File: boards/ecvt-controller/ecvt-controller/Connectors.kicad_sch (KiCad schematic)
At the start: 8 parts, among them J2 917782-1, J3 917782-1, J4 15311026, J5 917786-1, J6 917780-1

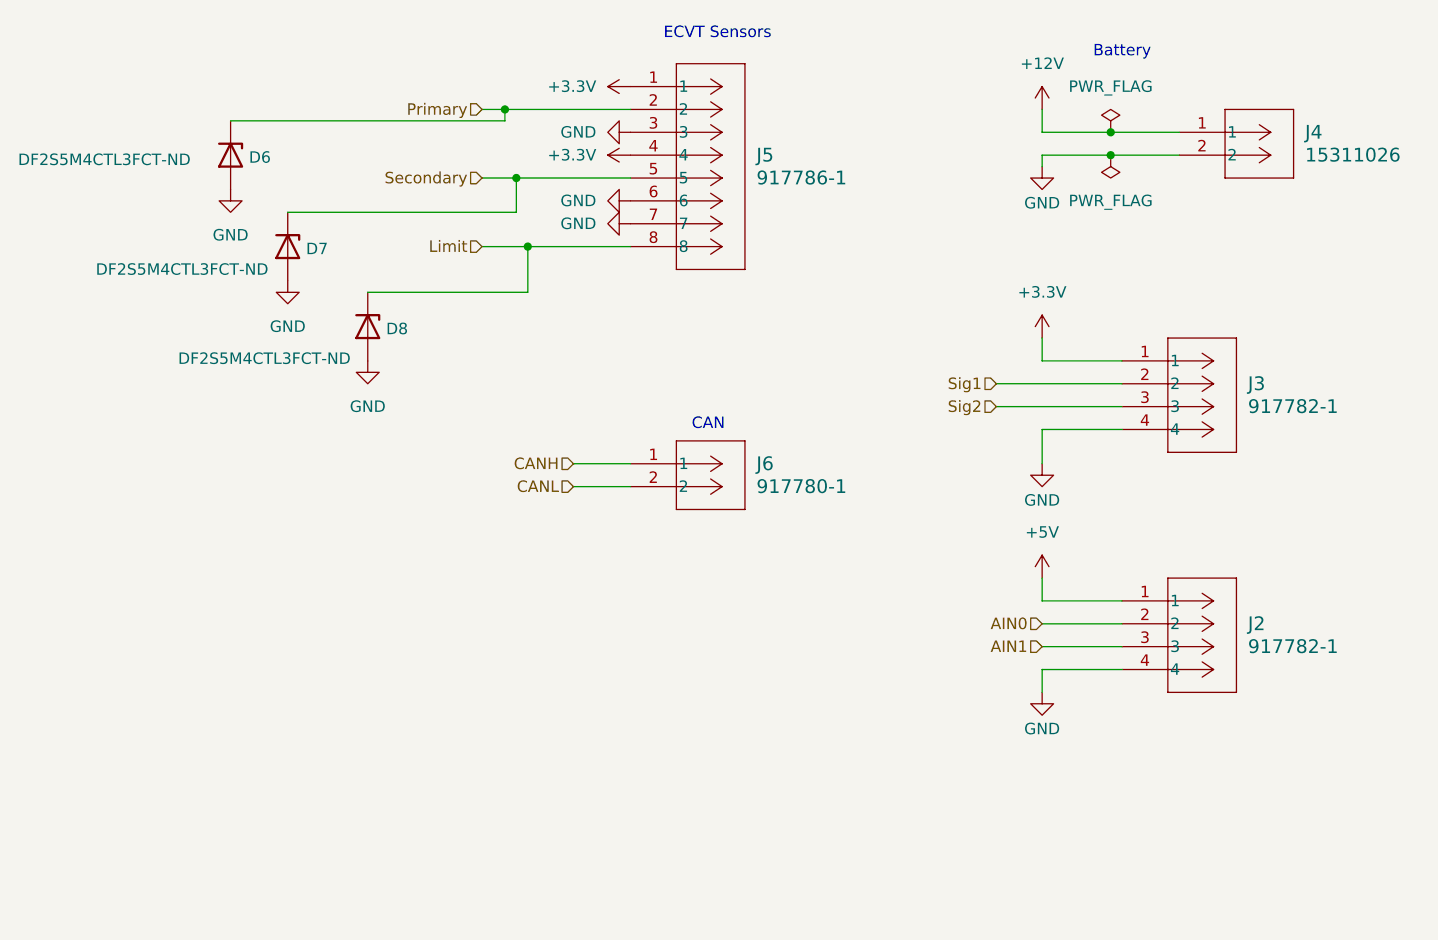
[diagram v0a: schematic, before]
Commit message: almost there
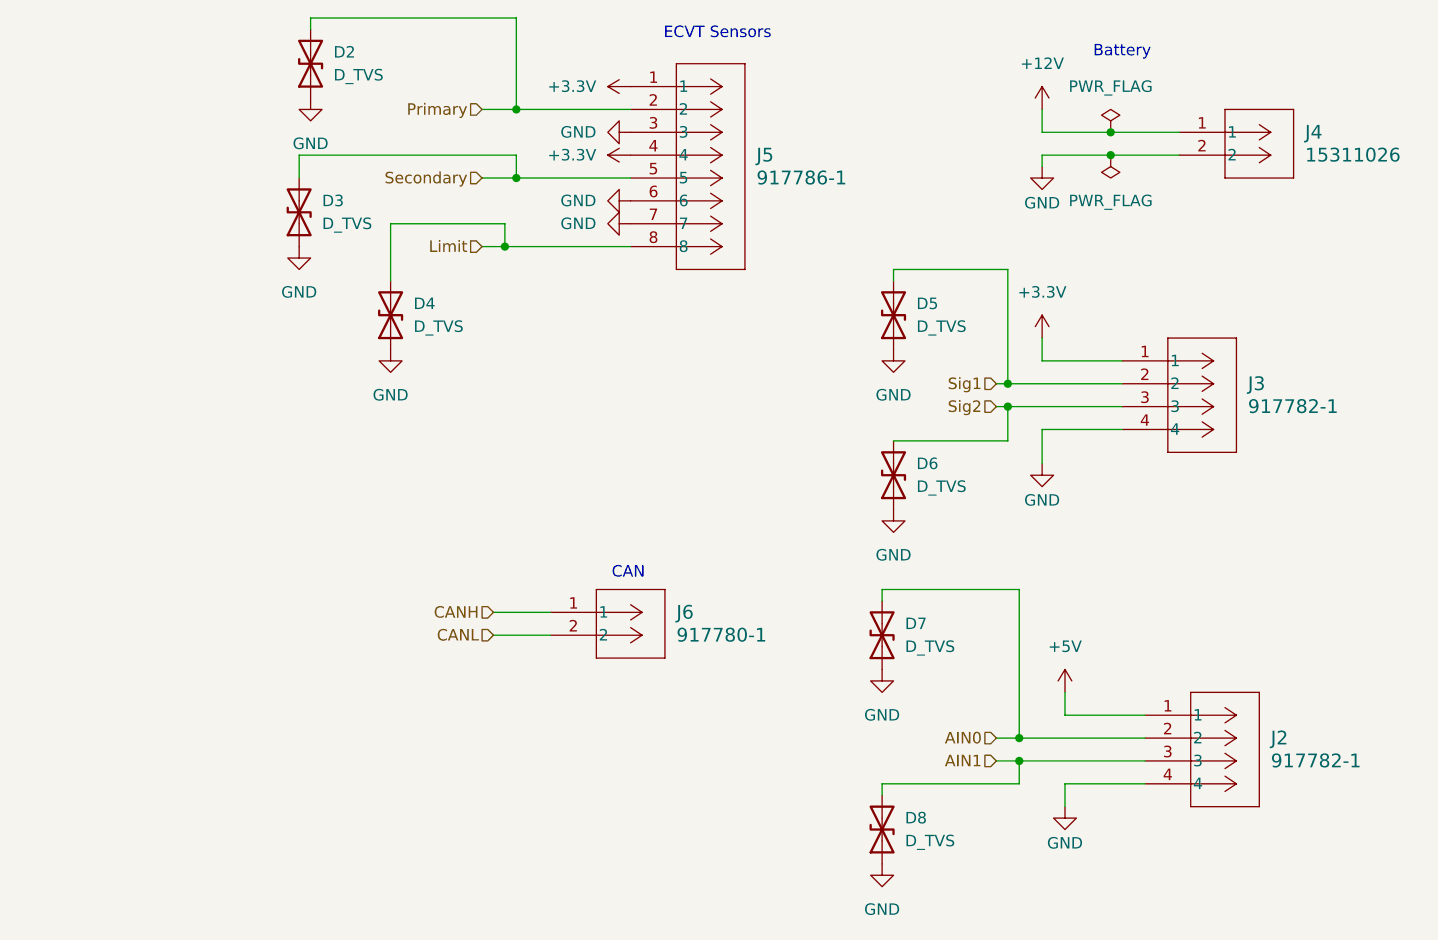
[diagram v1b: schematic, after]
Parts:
- removed D6, D7, D8: DF2S5M4CTL3FCT-ND, Diode_SMD:D_SOD-882, symbol Device:D_Zener
- added D2, D3, D4, D5, D6, D7, D8: D_TVS, Diode_SMD:D_SOD-323_HandSoldering, symbol Device:D_TVS
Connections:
- net AIN0: now also D7.2 (A2)
- net AIN1: now also D8.2 (A2)
- net GND: now also D2.1 (A1), D3.1 (A1), D4.1 (A1), D5.1 (A1), D6.1 (A1), D7.1 (A1), D8.1 (A1)
- net Limit: now also D4.2 (A2)
- net Primary: now also D2.2 (A2)
- net Secondary: now also D3.2 (A2)
- net Sig1: now also D5.2 (A2)
- net Sig2: now also D6.2 (A2)
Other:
- moved on the sheet: J2, J6
